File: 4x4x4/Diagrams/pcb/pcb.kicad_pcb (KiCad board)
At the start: 2 copper layers, 77 parts, among them J1 Conn_01x04_Female, J10 Conn_01x04_Female, J11 Conn_01x04_Female, J12 Conn_01x04_Female, J13 Conn_01x04_Female, J14 Conn_01x04_Female, J2 Conn_01x06_Female, J3 Conn_01x04_Female, J4 Conn_01x04_Female, J5 Conn_01x04_Female, J6 Conn_01x04_Female, J7 Conn_01x04_Female, J8 Conn_01x04_Female, J9 Conn_01x04_Female, Q1 2N2222, Q2 2N2222, Q3 2N2222, Q4 2N2222, U1 74HC595, U2 74HC595, U3 74HC595, U4 74HC595, U5 74HC595, U6 74HC595, U7 74HC595

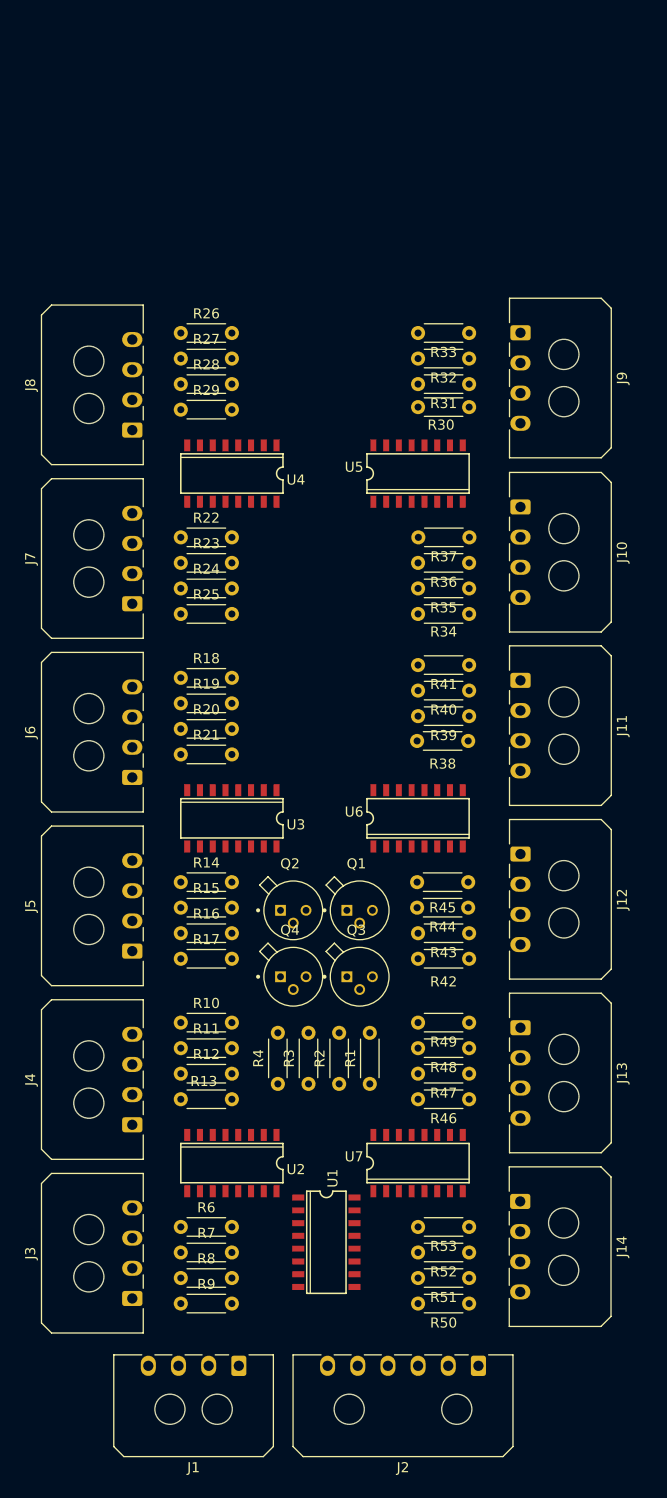
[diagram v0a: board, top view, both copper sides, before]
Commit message: layout pcb complete
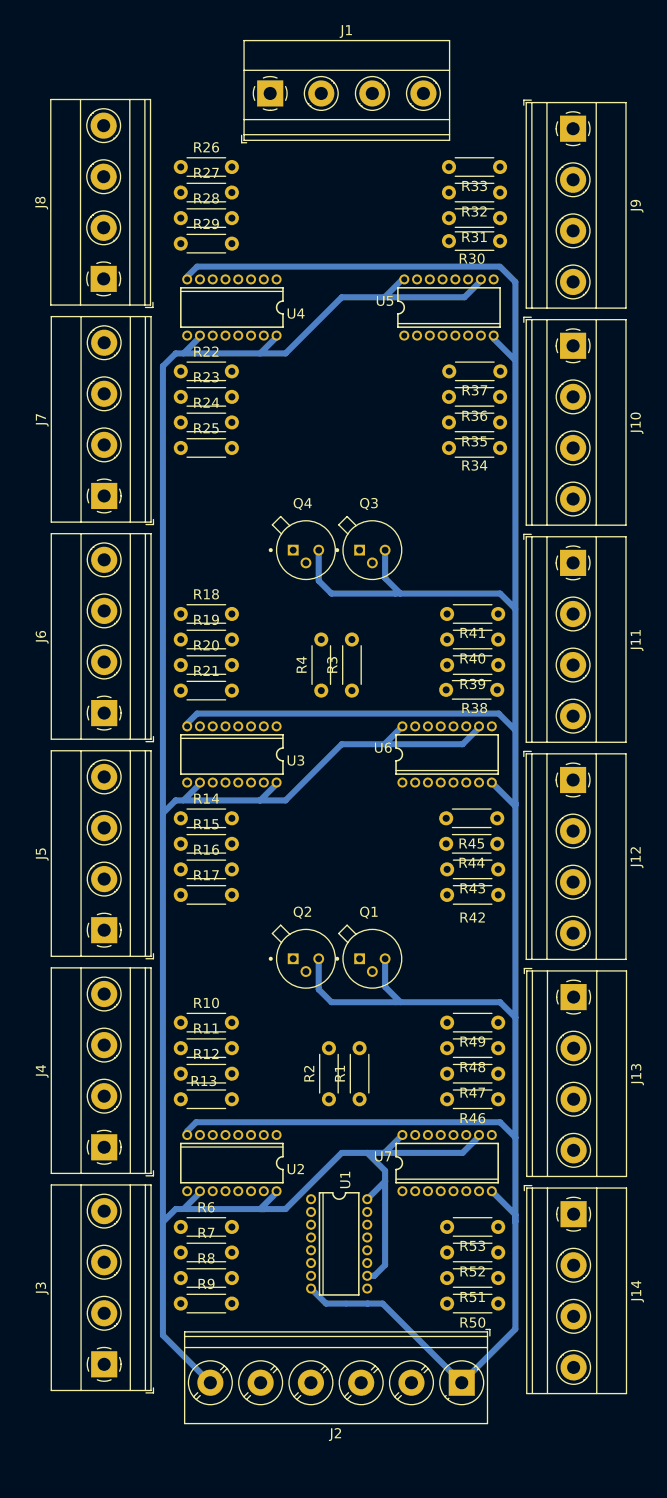
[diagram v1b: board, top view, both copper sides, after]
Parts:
- J1, J10, J11, J12, J13, J14, J3, J4, J5, J6, J7, J8, J9: footprint Connector_Molex:Molex_Micro-Fit_3.0_43650-0400_1x04_P3.00mm_Horizontal -> TerminalBlock_Phoenix:TerminalBlock_Phoenix_MKDS-1,5-4-5.08_1x04_P5.08mm_Horizontal
- J2: footprint Connector_Molex:Molex_Micro-Fit_3.0_43650-0600_1x06_P3.00mm_Horizontal -> TerminalBlock_Phoenix:TerminalBlock_Phoenix_PT-1,5-6-5.0-H_1x06_P5.00mm_Horizontal
- moved J1 126.6 mm to (78.7, 28.2), turned to 0 degrees
- moved Q3 42.4 mm to (88.9, 73.7)
- moved Q4 42.4 mm to (82.3, 73.7)
- moved R3 39.4 mm to (86.9, 87.6)
- moved R4 39.4 mm to (83.8, 87.6)
- moved J9 21.0 mm to (108.9, 31.8)
- moved J10 16.9 mm to (108.9, 53.3)
- moved U5 16.8 mm to (96.5, 49.5)
- moved R34 16.8 mm to (101.6, 63.5)
- moved R36 16.8 mm to (101.6, 58.4)
- moved R30 16.8 mm to (101.6, 42.9)
- moved R31 16.8 mm to (101.6, 40.6)
- moved R32 16.8 mm to (101.6, 38.1)
- moved R33 16.8 mm to (101.6, 35.6)
- moved R35 16.8 mm to (101.6, 61.0)
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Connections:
- Q1 pad 1: Net-(J1-Pad4) -> Net-(J1-Pad1)
- Q2 pad 1: Net-(J1-Pad3) -> Net-(J1-Pad2)
- Q3 pad 1: Net-(J1-Pad2) -> Net-(J1-Pad3)
- Q4 pad 1: Net-(J1-Pad1) -> Net-(J1-Pad4)
- R1 pad 2: Net-(Q4-Pad2) -> Net-(Q1-Pad2)
- R2 pad 2: Net-(Q3-Pad2) -> Net-(Q2-Pad2)
- R3 pad 2: Net-(Q2-Pad2) -> Net-(Q3-Pad2)
- R4 pad 2: Net-(Q1-Pad2) -> Net-(Q4-Pad2)
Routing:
- net GND: track 0.00 -> 300.4 mm
- net Net-(J2-Pad6): track 0.00 -> 246.8 mm
